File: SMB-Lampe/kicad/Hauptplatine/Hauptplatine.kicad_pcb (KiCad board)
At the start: 2 copper layers, 52 x 34 mm, 12 parts, among them J1 Screw_Terminal_01x02, J2 Screw_Terminal_01x02, J3 Screw_Terminal_01x02, J4 Screw_Terminal_01x02, J5 Screw_Terminal_01x02, J6 Screw_Terminal_01x02, U1 MOUDLE-SEEEDUINO-XIAO-ESP32C3, U2 4-Kanal-I2C Pegelwandler

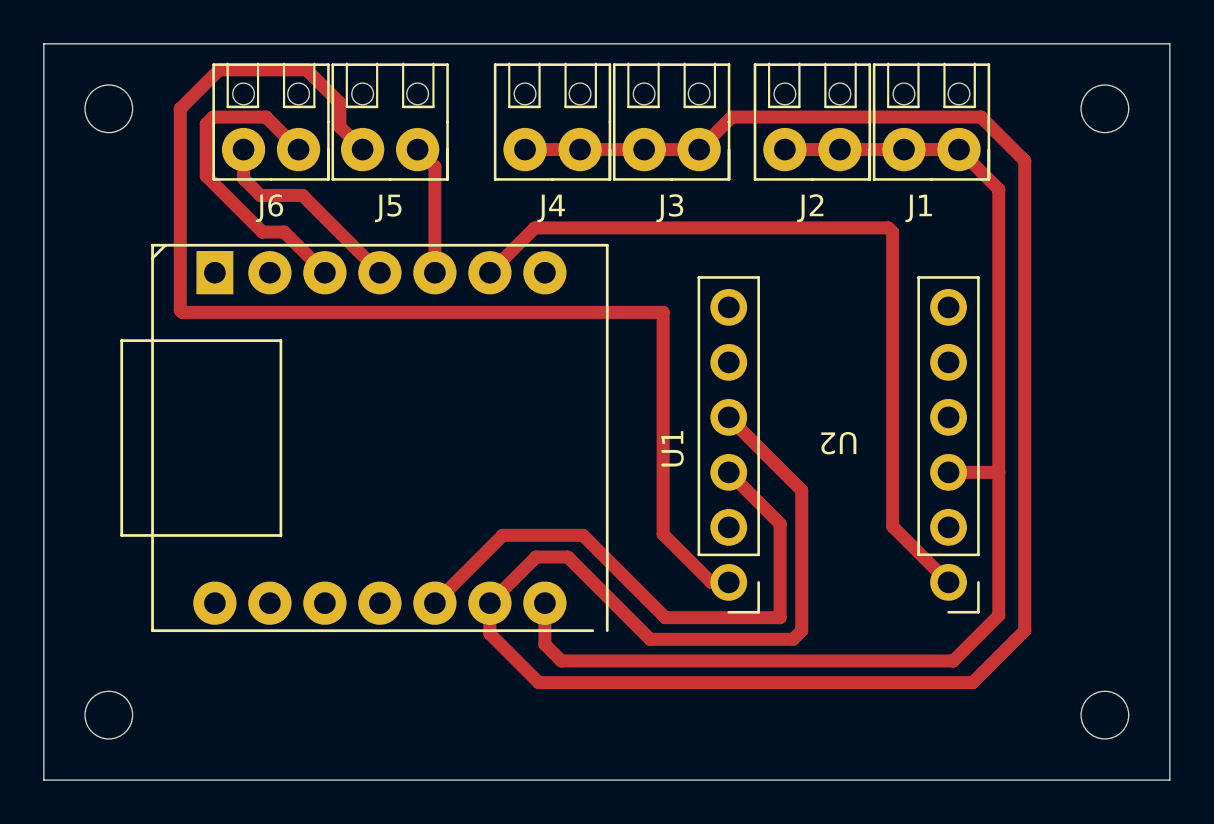
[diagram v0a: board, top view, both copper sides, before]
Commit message: Nachträgliche Änderungen für die Fertigung und Präsentation
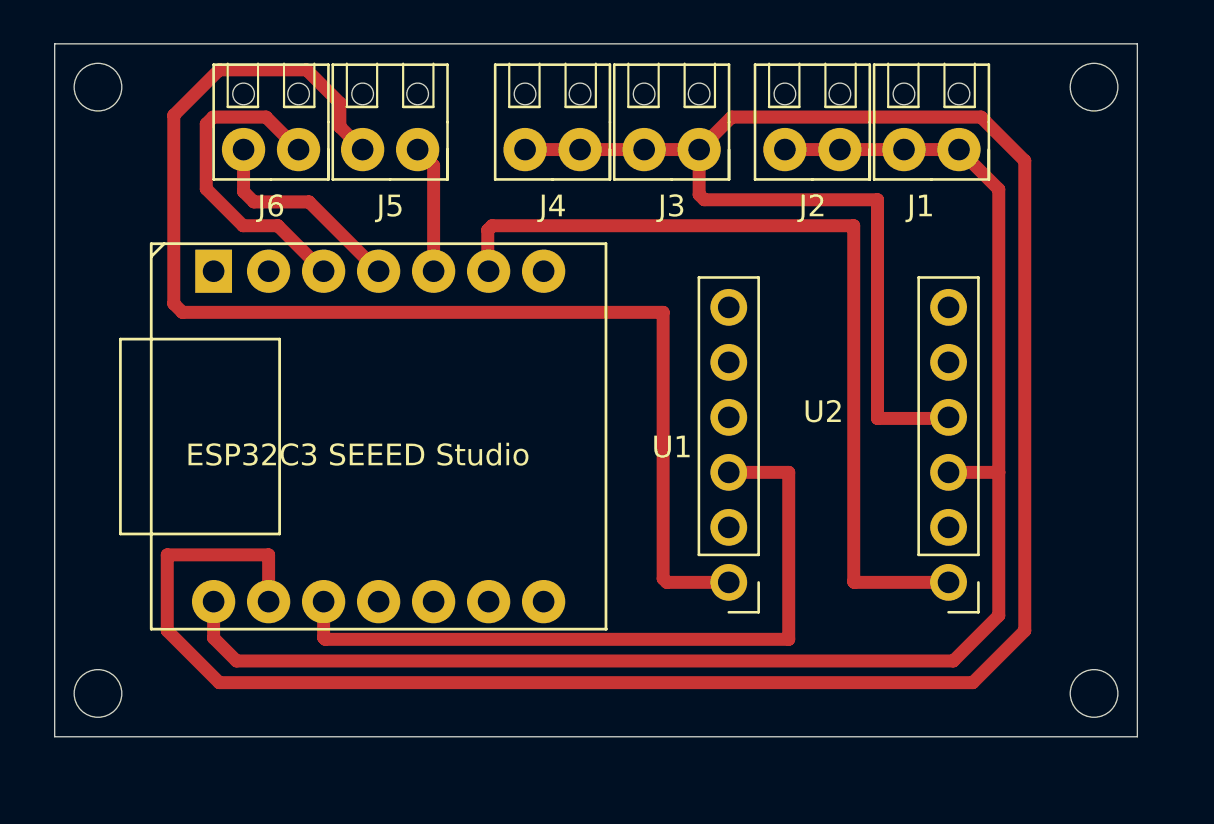
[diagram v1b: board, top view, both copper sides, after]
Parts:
- U1: value MOUDLE-SEEEDUINO-XIAO-ESP32C3 -> ESP32C3 SEEED Studio
- moved REF** 1.12 mm to (154.5, 109.0)
- moved REF** 1.12 mm to (154.5, 81.0)
- moved REF** 1.12 mm to (108.5, 109.0)
- moved REF** 1.12 mm to (108.5, 81.0)
- moved U1 0.09 mm to (132.0, 97.1)
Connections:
- net Daten_LED renamed Data_LED
- U2 pad 10: unconnected-(U2-GND-Pad10) -> GND
- U2 pad 4: GND -> unconnected-(U2-GND-Pad4)
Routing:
- net GND: track 102.5 -> 122.0 mm
- net +5V: track 56.7 -> 71.9 mm
- net +3.3V: track 26.5 -> 33.7 mm
- net Net-(U1-PA9_A5_D5_SCL): track 36.8 -> 39.7 mm
- net /ECHO_Ultraschall: track 57.2 -> 58.6 mm
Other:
- board size 52 x 34 mm -> 50 x 32 mm
